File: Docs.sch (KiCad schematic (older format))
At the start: 0 parts

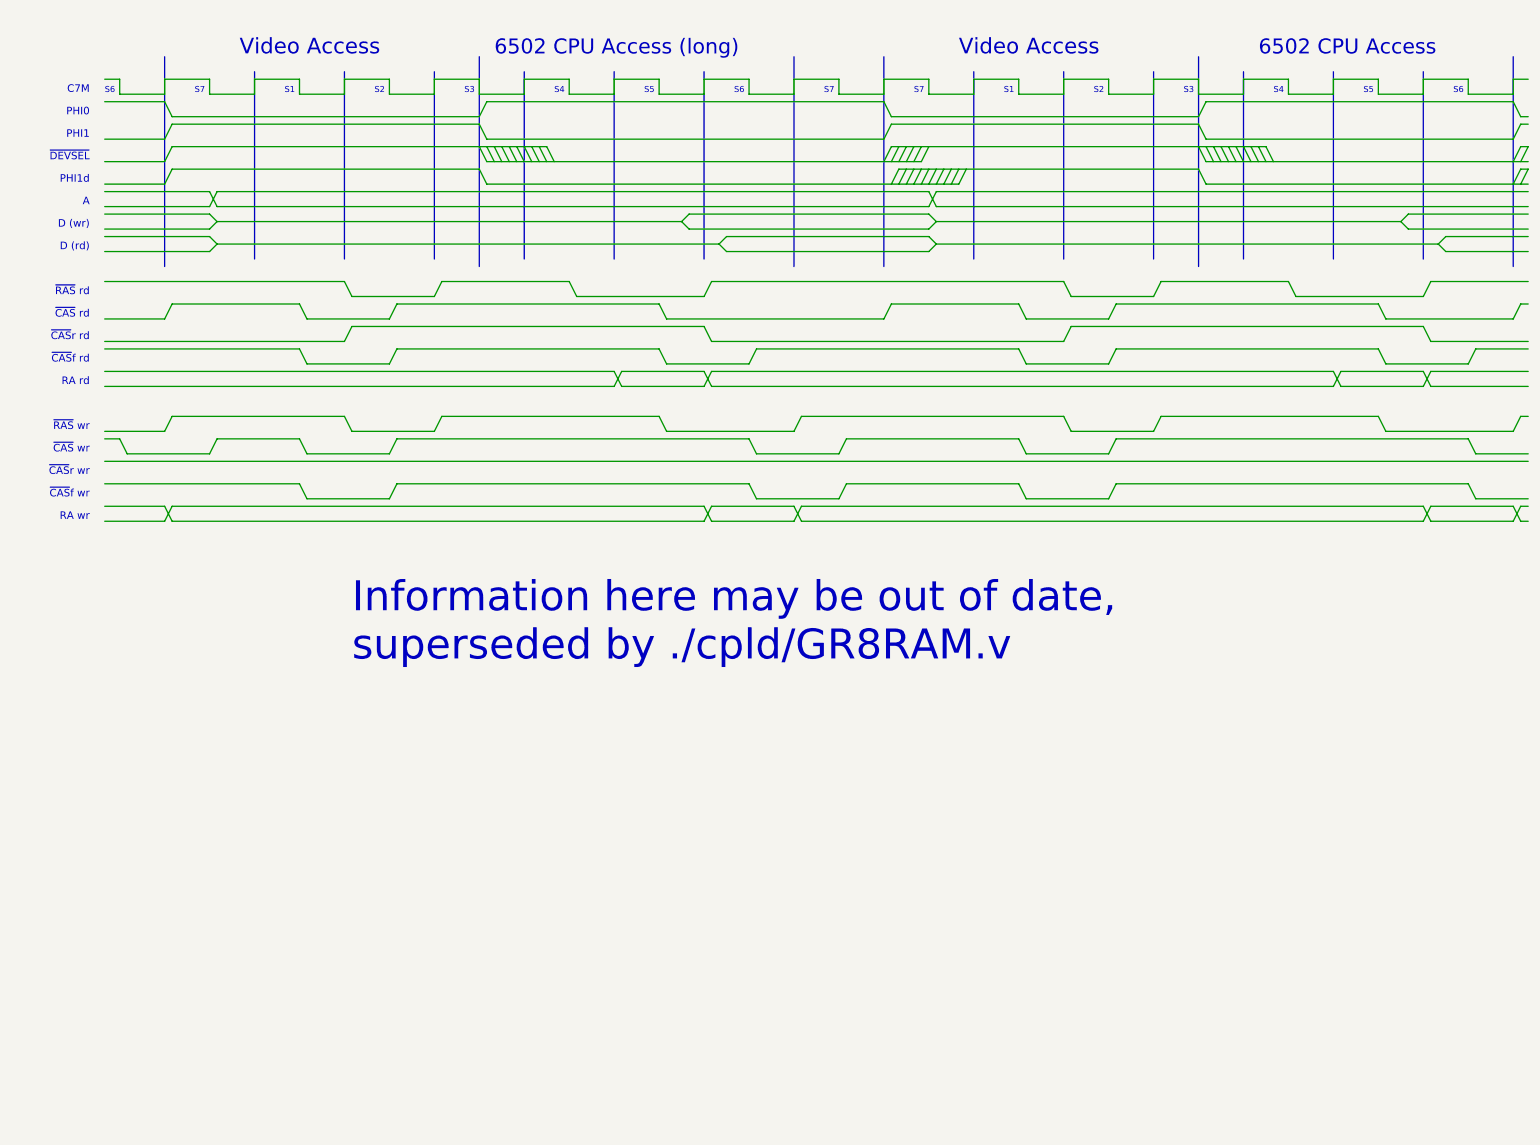
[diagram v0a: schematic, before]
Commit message: Board done?
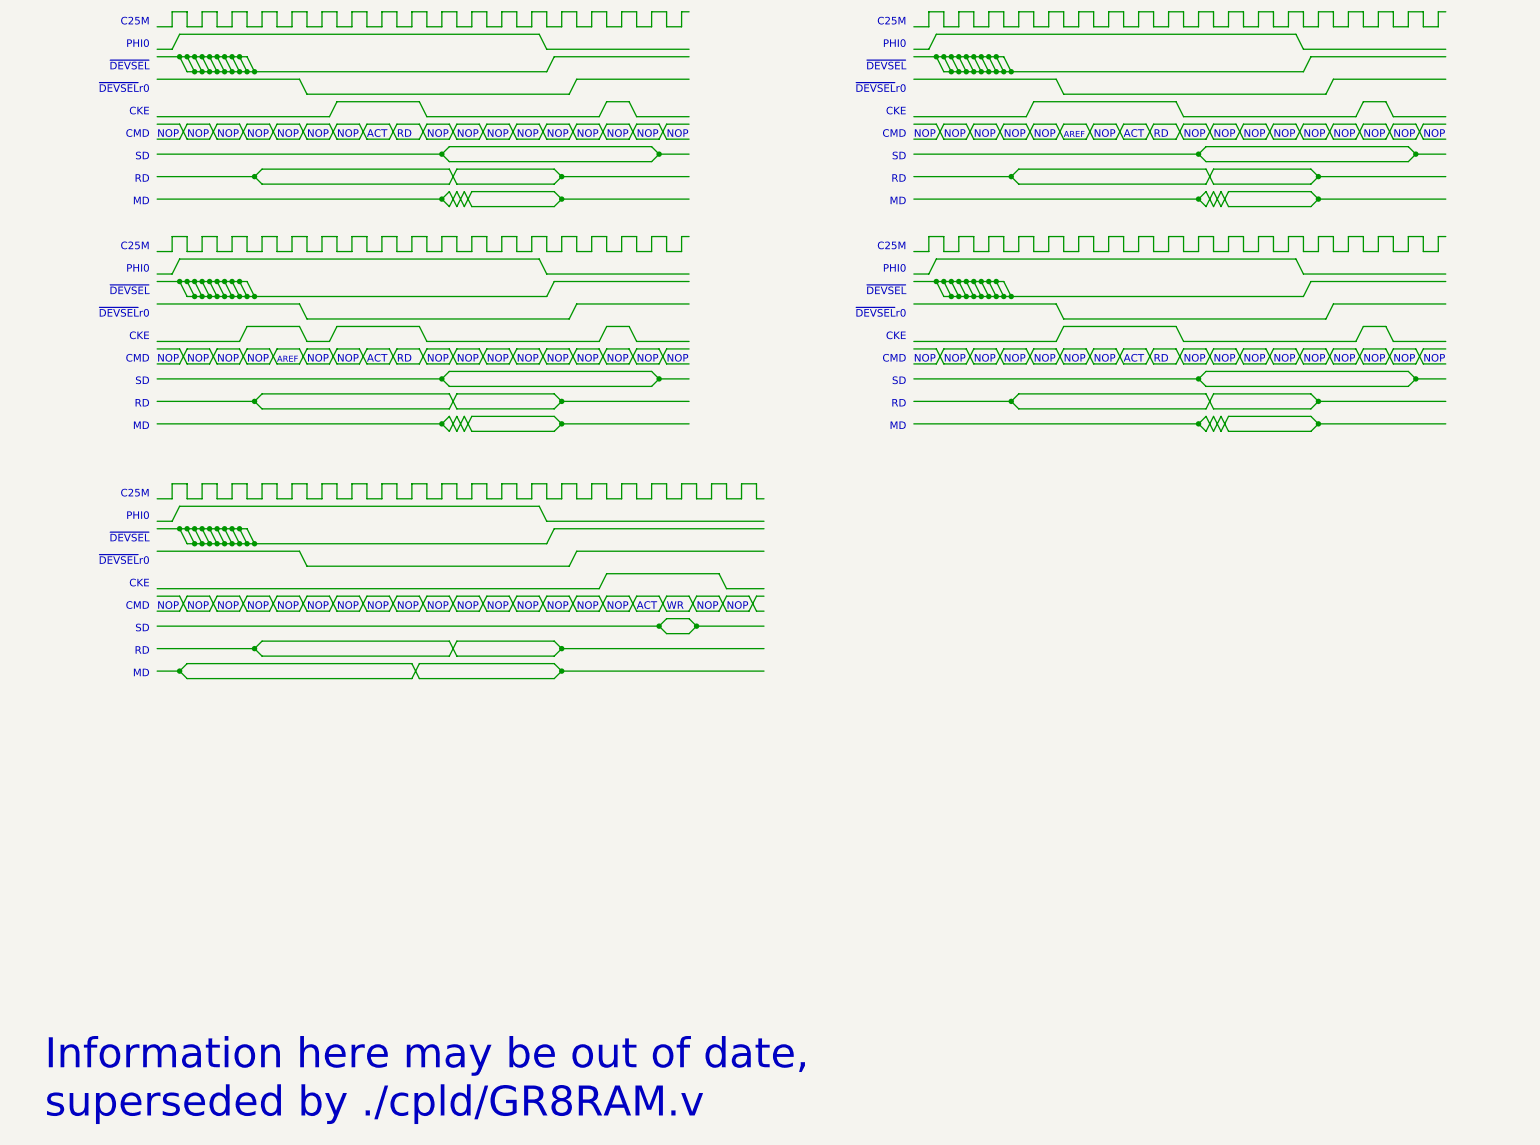
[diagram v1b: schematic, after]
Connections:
- wire segments 343 -> 1150
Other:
- note added: "ACT"
- note added: "AREF"
- note added: "C25M"
- note added: "CKE"
- note added: "CMD"
- note added: "MD"
- note added: "NOP"
- note added: "RD"
- note added: "SD"
- note added: "WR"
- note added: "~DEVSEL~r0"
- note removed: "6502 CPU Access"
- note removed: "6502 CPU Access (long)"
- note removed: "A"
- note removed: "C7M"
- note removed: "D (rd)"
- note removed: "D (wr)"
- note removed: "PHI1"
- note removed: "PHI1d"
- note removed: "RA rd"
- note removed: "RA wr"
- note removed: "S1"
- note removed: "S2"
- note removed: "S3"
- note removed: "S4"
- note removed: "S5"
- note removed: "S6"
- note removed: "S7"
- note removed: "Video Access"
- note removed: "~CAS~ rd"
- note removed: "~CAS~ wr"
- note removed: "~CAS~f rd"
- note removed: "~CAS~f wr"
- note removed: "~CAS~r rd"
- note removed: "~CAS~r wr"
- note removed: "~RAS~ rd"
- note removed: "~RAS~ wr"
